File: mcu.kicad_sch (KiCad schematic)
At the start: 32 parts, among them J4 Conn_02x05_Odd_Even, U7 STM32F407VGTx, U8 STM809SWX6F, Y1 8MHz

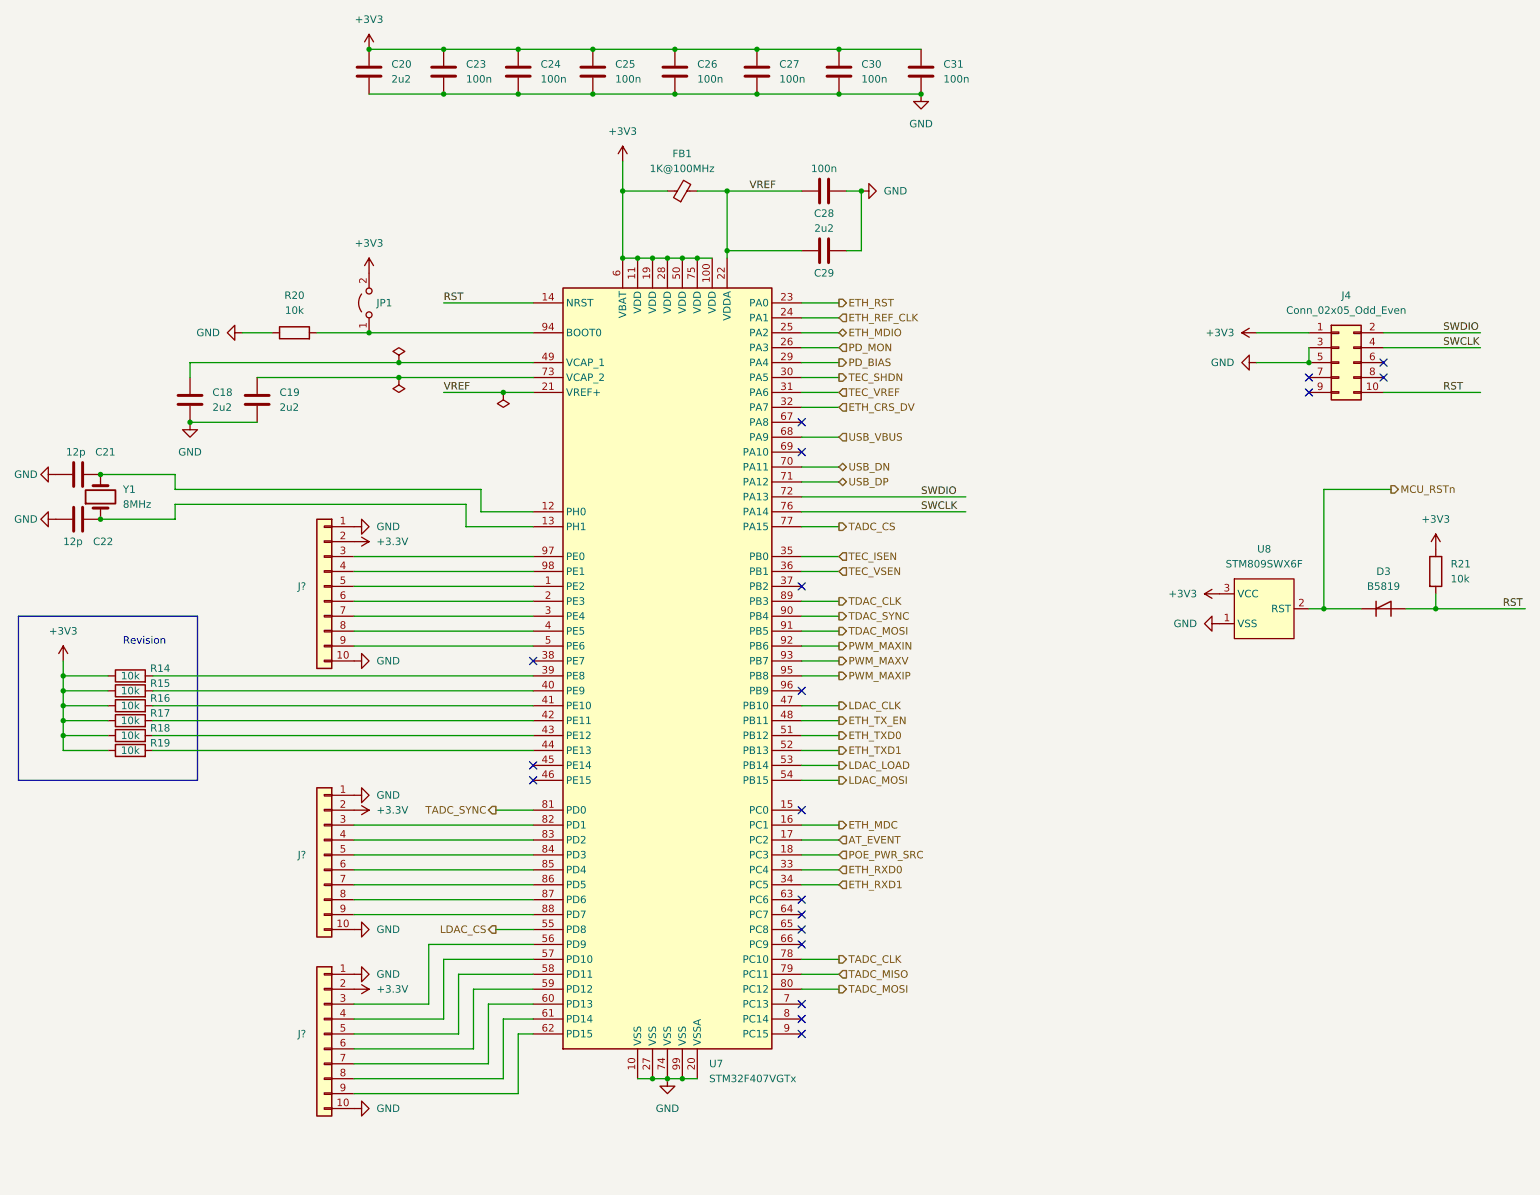
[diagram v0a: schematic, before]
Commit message: v 0.2 schematics
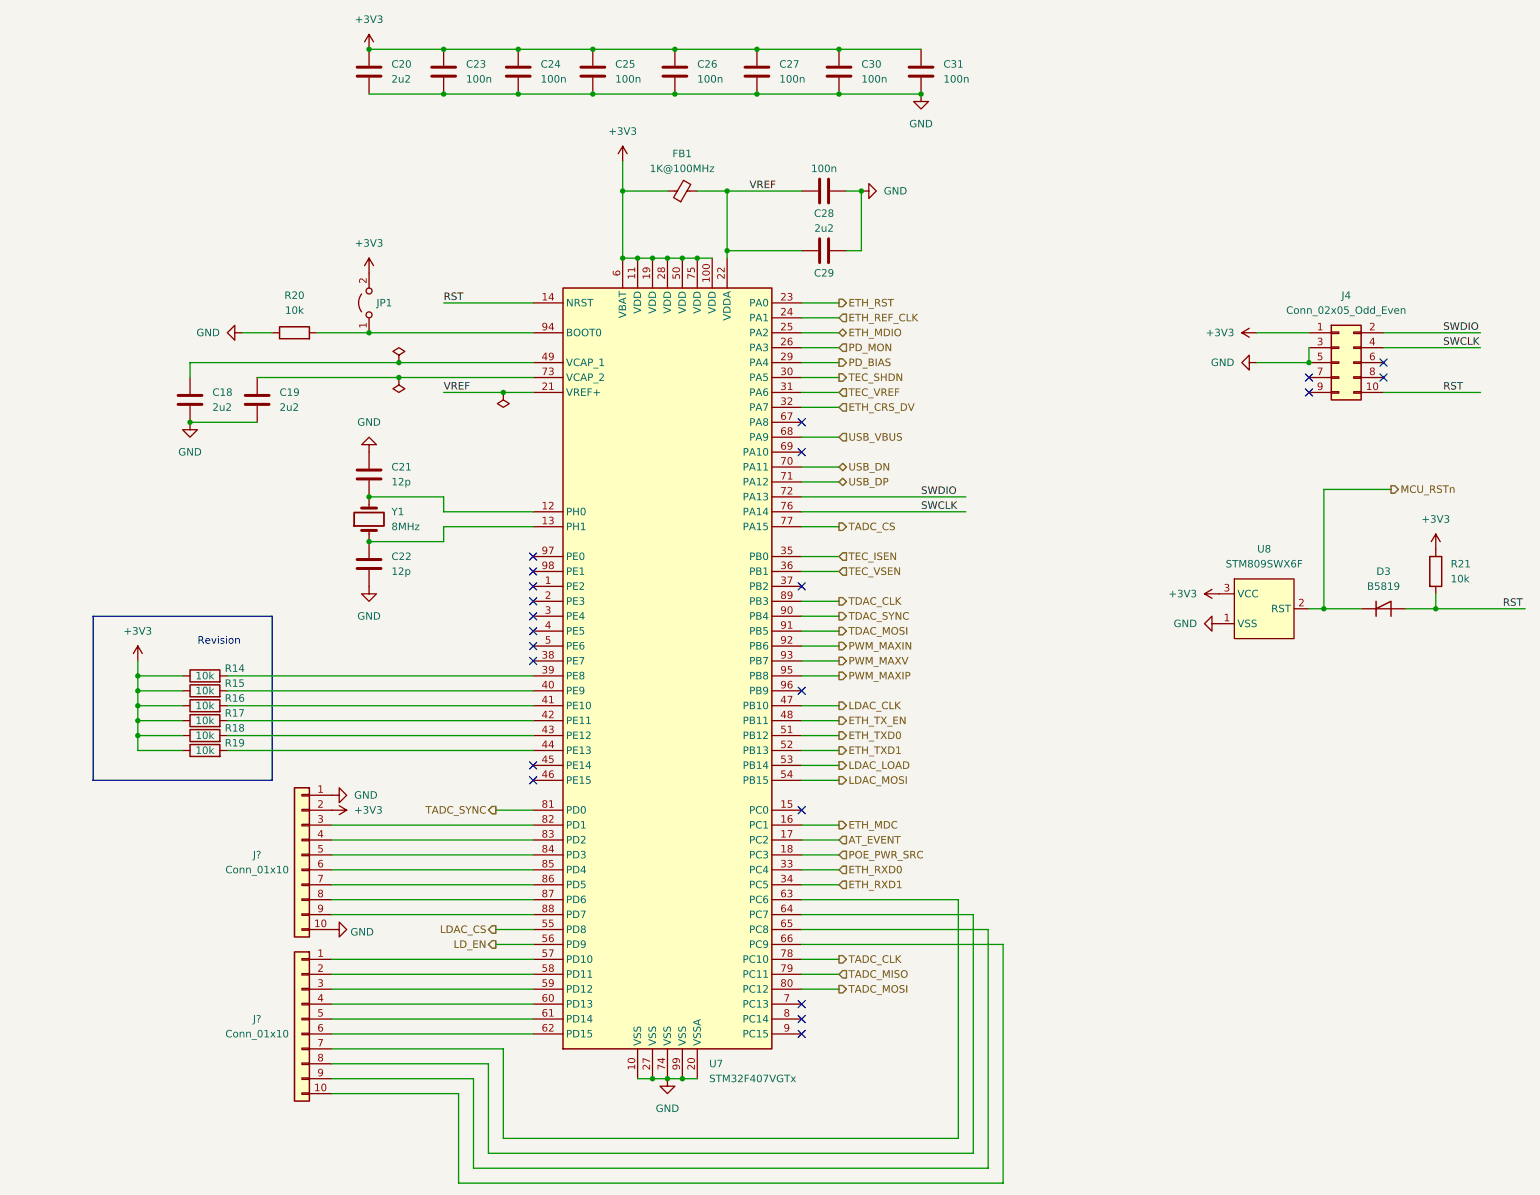
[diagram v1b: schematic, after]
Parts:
- removed J? (x3): Conn_01x10, symbol Connector_Generic:Conn_01x10
- added J? (x2): Conn_01x10, symbol Connector_Generic:Conn_01x10
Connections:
- net +3V3: now also J?.2 (Pin_2)
- net GND: now also J?.1 (Pin_1), J?.10 (Pin_10)
- net LD_EN: now reaches U7.56 (PD9)
- net at U7.57 (PD10): now also J?.1 (Pin_1)
- net at U7.58 (PD11): now also J?.2 (Pin_2)
- net at U7.59 (PD12): now also J?.3 (Pin_3)
- net at U7.60 (PD13): now also J?.4 (Pin_4)
- net at U7.61 (PD14): now also J?.5 (Pin_5)
- net at U7.62 (PD15): now also J?.6 (Pin_6)
- net at U7.63 (PC6): now also J?.7 (Pin_7)
- net at U7.64 (PC7): now also J?.8 (Pin_8)
- net at U7.65 (PC8): now also J?.9 (Pin_9)
- net at U7.66 (PC9): now also J?.10 (Pin_10)
- net at U7.82 (PD1): now also J?.3 (Pin_3)
- net at U7.83 (PD2): now also J?.4 (Pin_4)
- net at U7.84 (PD3): now also J?.5 (Pin_5)
- net at U7.85 (PD4): now also J?.6 (Pin_6)
- net at U7.86 (PD5): now also J?.7 (Pin_7)
- net at U7.87 (PD6): now also J?.8 (Pin_8)
- net at U7.88 (PD7): now also J?.9 (Pin_9)
- no-connect marks 19 -> 22
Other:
- moved on the sheet: C21, C22, R14, R15, R16, R17, R18, R19, Y1
